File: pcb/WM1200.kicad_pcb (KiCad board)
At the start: 4 copper layers, 147 x 104 mm, 143 parts, among them Q1 BC817, Q2 BC817, Q3 BC817, Q4 BC817, Q5 BC817, Q6 BC817, U1 74LVCH162245A, U2 74LVCH162245A, U3 74LVCH162245A, U4 74LVCH162245A, U5 74LVCH162245A, U6 ADP2108AUJ-3.3, U7 TPD12S016PWR, X1 audio_expansion, X2 A1200_trapdoor_connector, X3 AC7020, X4 Conn_02x05_Odd_Even, X5 HDMI_A

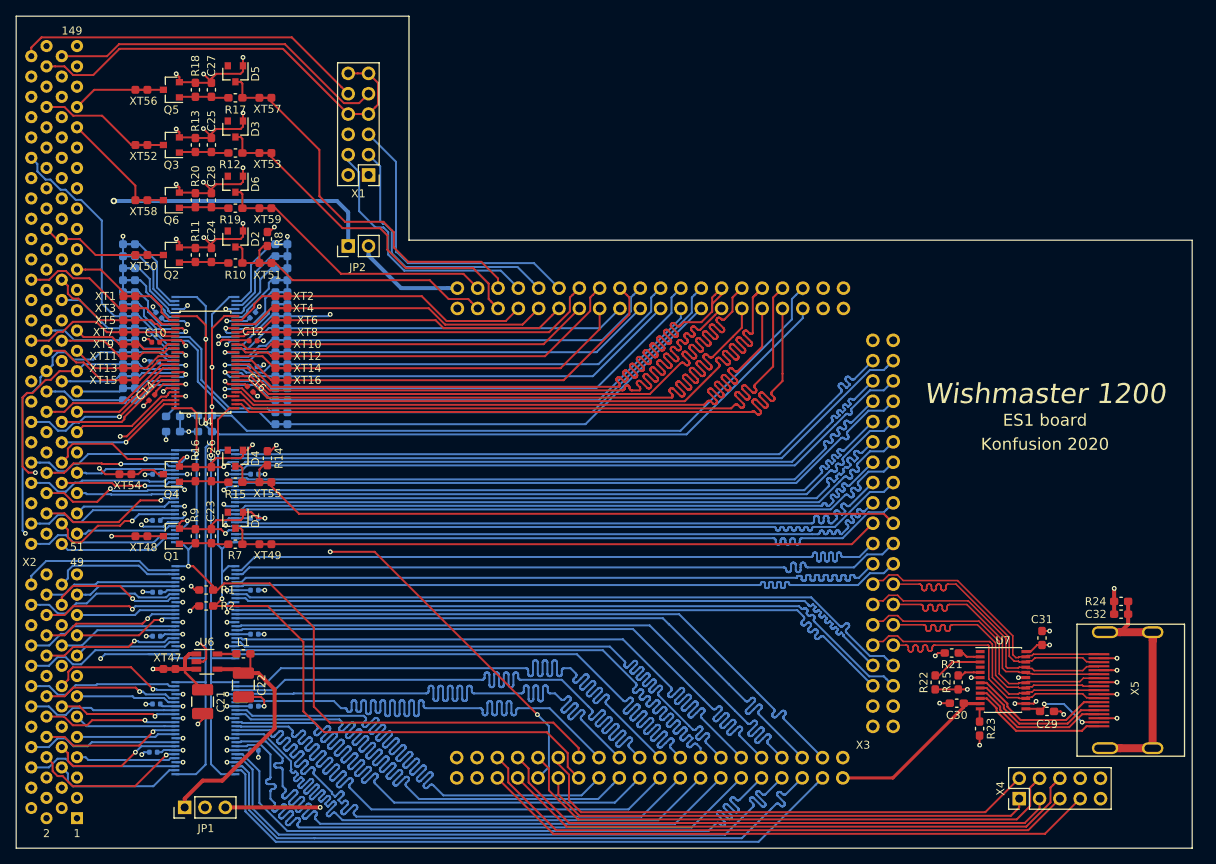
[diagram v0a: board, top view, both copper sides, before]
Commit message: factory DRC passed
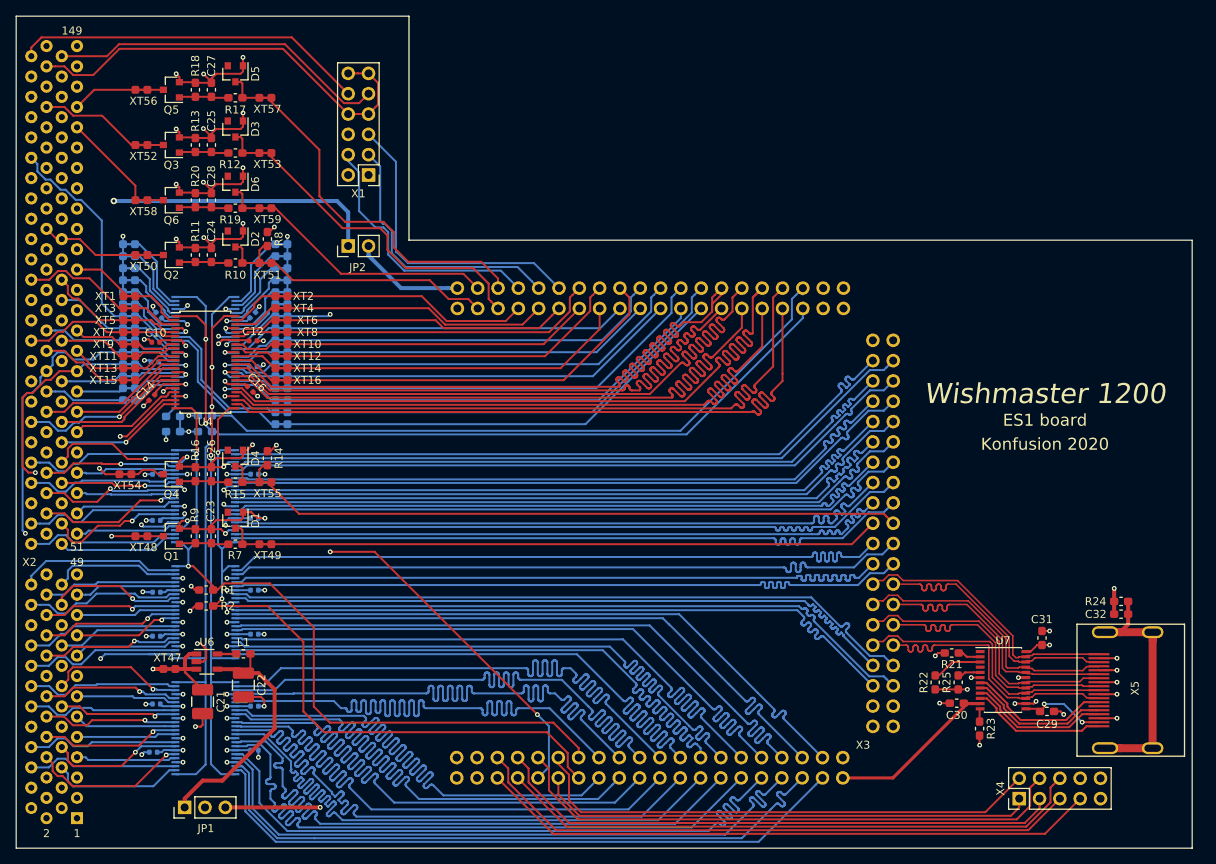
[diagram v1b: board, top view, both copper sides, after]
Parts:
- D1, D2, D3, D4, D5, D6: footprint Diode_SMD:D_SOT-23_ANK -> WM1200:D_SOT-23_ANK
- Q1, Q2, Q3, Q4, Q5, Q6: footprint Package_TO_SOT_SMD:SOT-23 -> WM1200:SOT-23
- U6: footprint Package_TO_SOT_SMD:TSOT-23-5 -> WM1200:TSOT-23-5
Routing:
- net GND: track 209.9 -> 210.8 mm
